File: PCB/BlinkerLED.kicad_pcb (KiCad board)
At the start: 2 copper layers, 99.1 x 99.1 mm, 19 parts, among them J1 Conn_01x02_Socket, J2 Conn_01x01_Socket, U1 NE555P, U2 4017

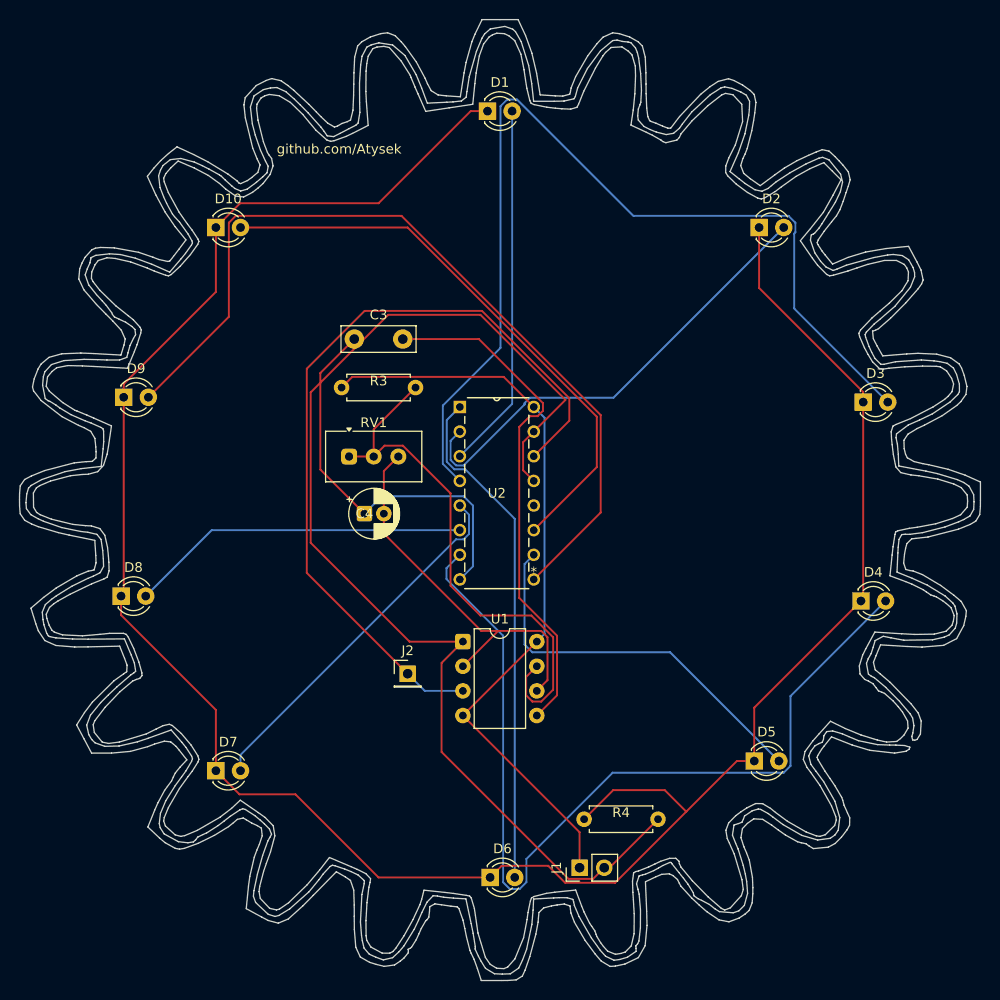
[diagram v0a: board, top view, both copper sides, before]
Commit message: Add files via upload
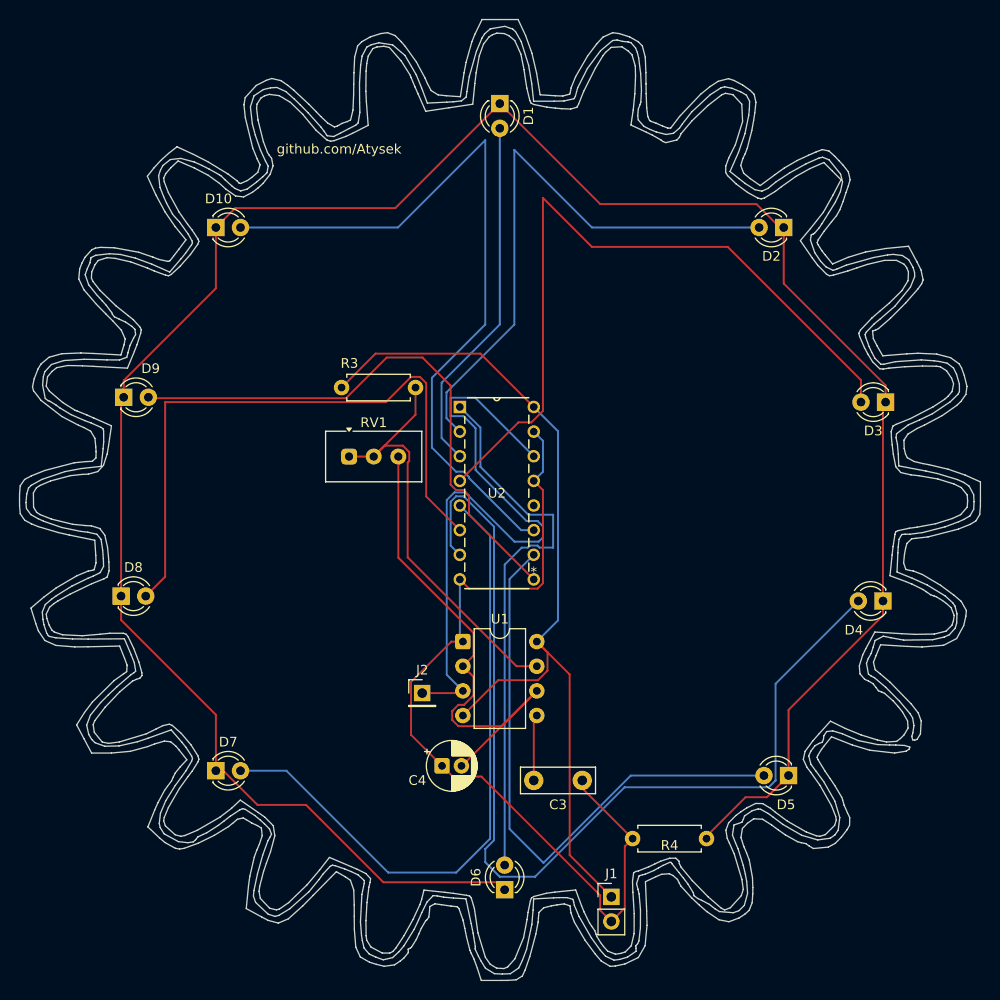
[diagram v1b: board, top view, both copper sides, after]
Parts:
- moved C3 51.2 mm to (117.5, 130.5), turned to 180 degrees
- moved C4 27.2 mm to (103.0, 129.0)
- moved R4 12.8 mm to (130.3, 136.5), turned to 180 degrees
- moved J1 4.44 mm to (120.5, 142.5), turned to 0 degrees
- moved D5 3.84 mm to (138.8, 130.0), turned to 180 degrees
- moved D2 2.54 mm to (138.3, 73.5), turned to 180 degrees
- moved J2 2.50 mm to (101.0, 121.5)
- moved D3 2.31 mm to (148.8, 91.5), turned to 180 degrees
- moved D4 2.27 mm to (148.5, 112.0), turned to 180 degrees
- moved D6 1.97 mm to (109.5, 141.8), turned to 90 degrees
- moved D1 1.49 mm to (109.0, 60.7), turned to -90 degrees
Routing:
- net GND: track 164.2 -> 92.2 mm
- net Net-(U1-CONT): track 53.3 -> 6.82 mm
- net Net-(D8-A): track 35.2 -> 65.7 mm
- net Net-(D9-A): track 88.4 -> 58.1 mm
- net Net-(D7-A): track 38.0 -> 67.2 mm
- net Net-(D3-A): track 100.3 -> 76.3 mm
- net Net-(D5-A): track 40.8 -> 60.7 mm
- net Net-(D10-A): track 59.2 -> 77.0 mm
- net +5V: track 78.0 -> 93.3 mm
- net OUT: track 82.9 -> 68.0 mm
- net TR: track 41.0 -> 54.0 mm
- net Net-(D2-A): track 48.1 -> 61.1 mm
- net Net-(U1-DISCH): track 56.6 -> 44.7 mm
- net Net-(D4-A): track 94.4 -> 103.5 mm
- net Net-(D6-A): track 52.6 -> 56.9 mm
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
